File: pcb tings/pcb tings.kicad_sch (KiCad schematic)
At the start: 24 parts, among them SW1 SW_Push, U1 ATmega32U4-A, Y1 16MHz

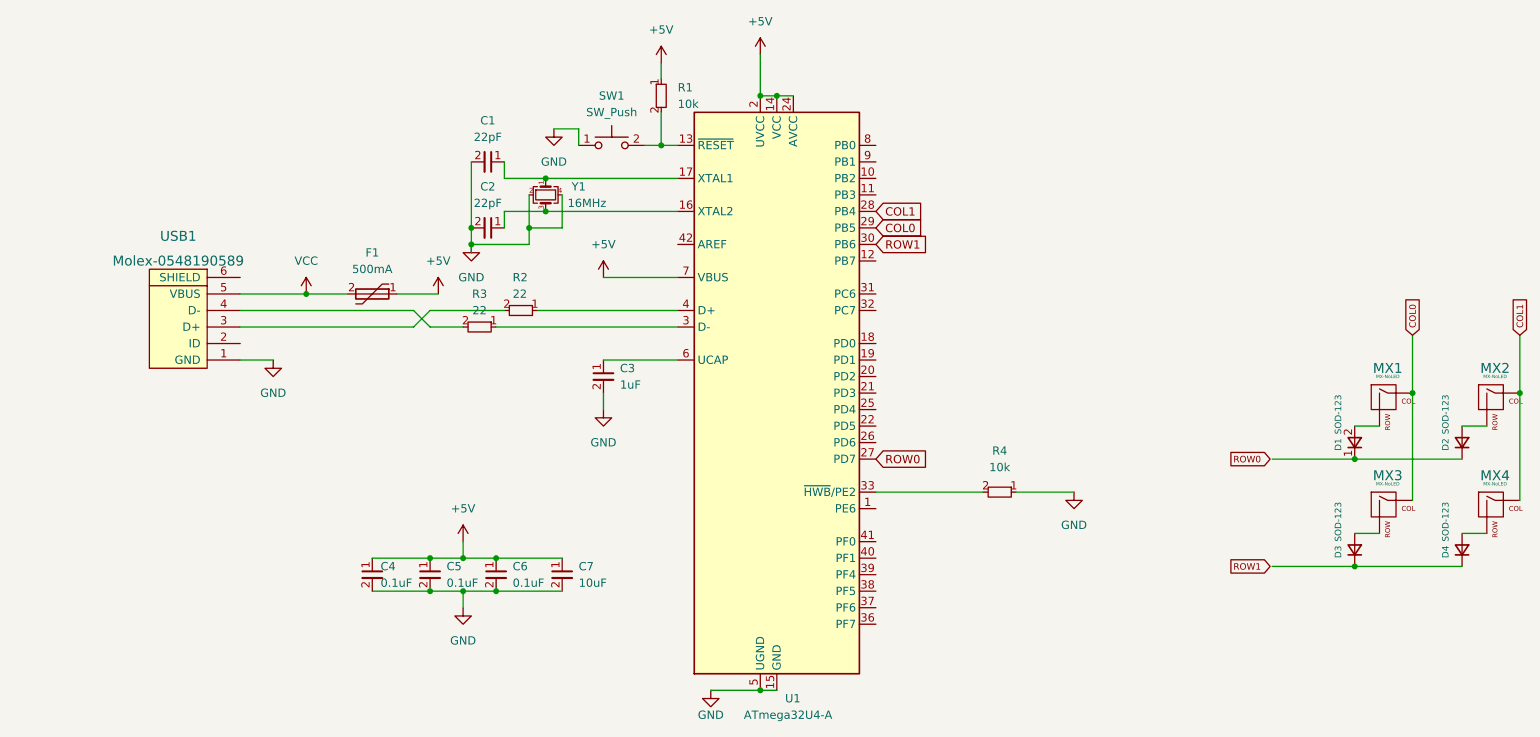
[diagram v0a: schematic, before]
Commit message: Routing
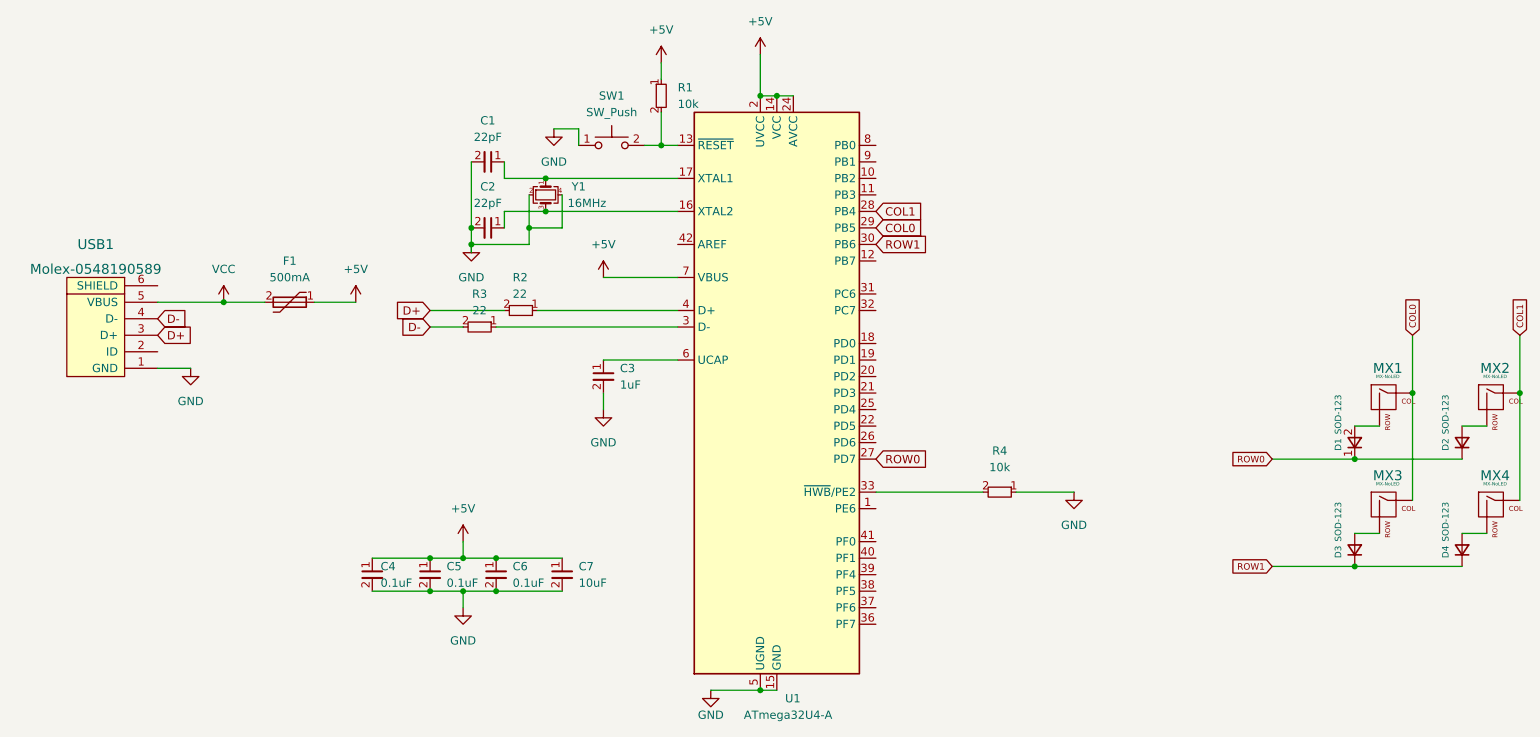
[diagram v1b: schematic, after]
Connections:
- net ROW0: now also D1.1 (K), D2.1 (K)
- net ROW1: now also D3.1 (K), D4.1 (K)
- net D+: now reaches USB1.3 (D+)
- net D+: now also R2.2
- net D-: now reaches USB1.4 (D-)
- net D-: now also R3.2
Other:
- moved on the sheet: F1, USB1
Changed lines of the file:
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@@
   (junction (at 127 48.26) (diameter 0) (color 0 0 0 0)
   )
-  (junction (at 57.15 78.74) (diameter 0) (color 0 0 0 0)
+  (junction (at 44.45 80.01) (diameter 0) (color 0 0 0 0)
   )
   (junction (at 227.33 93.98) (diameter 0) (color 0 0 0 0)
@@
   (junction (at 76.2 124.46) (diameter 0) (color 0 0 0 0)
   )
-  (bus_entry (at 76.2 83.82) (size -2.54 -2.54)
-    (stroke (width 0) (type default) (color 0 0 0 0))
-  )
-  (bus_entry (at 73.66 83.82) (size 2.54 -2.54)
-    (stroke (width 0) (type default) (color 0 0 0 0))
-  )
   (wire (pts (xy 92.71 81.28) (xy 114.3 81.28))
     (stroke (width 0) (type default) (color 0 0 0 0))
@@
     (stroke (width 0) (type default) (color 0 0 0 0))
   )
-  (wire (pts (xy 46.99 78.74) (xy 57.15 78.74))
+  (wire (pts (xy 34.29 80.01) (xy 44.45 80.01))
     (stroke (width 0) (type default) (color 0 0 0 0))
   )
@@
     (stroke (width 0) (type default) (color 0 0 0 0))
   )
-  (wire (pts (xy 46.99 81.28) (xy 73.66 81.28))
-    (stroke (width 0) (type default) (color 0 0 0 0))
-  )
   (wire (pts (xy 111.76 50.8) (xy 111.76 55.88))
     (stroke (width 0) (type default) (color 0 0 0 0))
@@
     (stroke (width 0) (type default) (color 0 0 0 0))
   )
-  (wire (pts (xy 57.15 78.74) (xy 63.5 78.74))
+  (wire (pts (xy 44.45 80.01) (xy 50.8 80.01))
     (stroke (width 0) (type default) (color 0 0 0 0))
   )
@@
     (stroke (width 0) (type default) (color 0 0 0 0))
   )
-  (wire (pts (xy 46.99 83.82) (xy 73.66 83.82))
-    (stroke (width 0) (type default) (color 0 0 0 0))
-  )
   (wire (pts (xy 218.44 120.65) (xy 234.95 120.65))
     (stroke (width 0) (type default) (color 0 0 0 0))
@@
     (stroke (width 0) (type default) (color 0 0 0 0))
   )
-  (wire (pts (xy 71.12 78.74) (xy 77.47 78.74))
+  (wire (pts (xy 58.42 80.01) (xy 64.77 80.01))
     (stroke (width 0) (type default) (color 0 0 0 0))
   )
@@
     (stroke (width 0) (type default) (color 0 0 0 0))
   )
-  (wire (pts (xy 46.99 88.9) (xy 52.07 88.9))
+  (wire (pts (xy 34.29 90.17) (xy 39.37 90.17))
     (stroke (width 0) (type default) (color 0 0 0 0))
   )
@@
   (wire (pts (xy 93.98 60.96) (xy 114.3 60.96))
     (stroke (width 0) (type default) (color 0 0 0 0))
+  )
+  (global_label "D-" (shape input) (at 34.29 82.55 0) (fields_autoplaced)
+    (effects (font (size 1.27 1.27)) (justify left))
+    (property "Intersheet References" "${INTERSHEET_REFS}" (id 0) (at 39.5455 82.4706 0)
+      (effects (font (size 1.27 1.27)) (justify left) hide)
+    )
   )
   (global_label "COL0" (shape input) (at 227.33 85.09 90) (fields_autoplaced)
@@
     )
   )
+  (global_label "D+" (shape input) (at 34.29 85.09 0) (fields_autoplaced)
+    (effects (font (size 1.27 1.27)) (justify left))
+    (property "Intersheet References" "${INTERSHEET_REFS}" (id 0) (at 39.5455 85.0106 0)
+      (effects (font (size 1.27 1.27)) (justify left) hide)
+    )
+  )
   (global_label "ROW0" (shape input) (at 144.78 104.14 0) (fields_autoplaced)
     (effects (font (size 1.27 1.27)) (justify left))
@@
     )
   )
-  (global_label "ROW1" (shape output) (at 199.39 120.65 0) (fields_autoplaced)
-    (effects (font (size 1 1)) (justify left))
-    (property "Intersheet References" "${INTERSHEET_REFS}" (id 0) (at 205.4329 120.5875 0)
-      (effects (font (size 1 1)) (justify left) hide)
-    )
-  )
-  (global_label "ROW0" (shape output) (at 199.39 104.14 0) (fields_autoplaced)
-    (effects (font (size 1 1)) (justify left))
-    (property "Intersheet References" "${INTERSHEET_REFS}" (id 0) (at 205.4329 104.0775 0)
-      (effects (font (size 1 1)) (justify left) hide)
+  (global_label "D-" (shape input) (at 76.2 83.82 180) (fields_autoplaced)
+    (effects (font (size 1.27 1.27)) (justify right))
+    (property "Intersheet References" "${INTERSHEET_REFS}" (id 0) (at 70.9445 83.7406 0)
+      (effects (font (size 1.27 1.27)) (justify right) hide)
+    )
+  )
+  (global_label "ROW1" (shape input) (at 205.74 120.65 180) (fields_autoplaced)
+    (effects (font (size 1 1)) (justify right))
+    (property "Intersheet References" "${INTERSHEET_REFS}" (id 0) (at 199.6971 120.5875 0)
+      (effects (font (size 1 1)) (justify right) hide)
+    )
+  )
+  (global_label "D+" (shape input) (at 76.2 81.28 180) (fields_autoplaced)
+    (effects (font (size 1.27 1.27)) (justify right))
+    (property "Intersheet References" "${INTERSHEET_REFS}" (id 0) (at 70.9445 81.2006 0)
+      (effects (font (size 1.27 1.27)) (justify right) hide)
+    )
+  )
+  (global_label "ROW0" (shape input) (at 205.74 104.14 180) (fields_autoplaced)
+    (effects (font (size 1 1)) (justify right))
+    (property "Intersheet References" "${INTERSHEET_REFS}" (id 0) (at 199.6971 104.0775 0)
+      (effects (font (size 1 1)) (justify right) hide)
     )
   )
@@
     (pin "1")
   )
-  (symbol (lib_id "Device:Polyfuse") (at 67.31 78.74 270) (unit 1)
-    (in_bom yes) (on_board yes) (fields_autoplaced)
-    (property "Reference" "F1" (id 0) (at 67.31 72.39 90))
-    (property "Value" "500mA" (id 1) (at 67.31 74.93 90))
-    (property "Footprint" "Fuse:Fuse_1206_3216Metric" (id 2) (at 62.23 80.01 0)
+  (symbol (lib_id "Device:Polyfuse") (at 54.61 80.01 270) (unit 1)
+    (in_bom yes) (on_board yes) (fields_autoplaced)
+    (property "Reference" "F1" (id 0) (at 54.61 73.66 90))
+    (property "Value" "500mA" (id 1) (at 54.61 76.2 90))
+    (property "Footprint" "Fuse:Fuse_1206_3216Metric" (id 2) (at 49.53 81.28 0)
       (effects (font (size 1.27 1.27)) (justify left) hide)
     )
-    (property "Datasheet" "~" (id 3) (at 67.31 78.74 0)
+    (property "Datasheet" "~" (id 3) (at 54.61 80.01 0)
       (effects (font (size 1.27 1.27)) hide)
     )
@@
     (pin "4")
   )
-  (symbol (lib_id "power:+5V") (at 77.47 78.74 0) (unit 1)
-    (in_bom yes) (on_board yes) (fields_autoplaced)
-    (property "Reference" "#PWR05" (id 0) (at 77.47 82.55 0)
-      (effects (font (size 1.27 1.27)) hide)
-    )
-    (property "Value" "+5V" (id 1) (at 77.47 73.66 0))
-    (property "Footprint" "" (id 2) (at 77.47 78.74 0)
-      (effects (font (size 1.27 1.27)) hide)
-    )
-    (property "Datasheet" "" (id 3) (at 77.47 78.74 0)
-      (effects (font (size 1.27 1.27)) hide)
-    )
-    (pin "1")
-  )
-  (symbol (lib_id "power:VCC") (at 57.15 78.74 0) (unit 1)
-    (in_bom yes) (on_board yes) (fields_autoplaced)
-    (property "Reference" "#PWR04" (id 0) (at 57.15 82.55 0)
-      (effects (font (size 1.27 1.27)) hide)
-    )
-    (property "Value" "VCC" (id 1) (at 57.15 73.66 0))
-    (property "Footprint" "" (id 2) (at 57.15 78.74 0)
-      (effects (font (size 1.27 1.27)) hide)
-    )
-    (property "Datasheet" "" (id 3) (at 57.15 78.74 0)
+  (symbol (lib_id "power:+5V") (at 64.77 80.01 0) (unit 1)
+    (in_bom yes) (on_board yes) (fields_autoplaced)
+    (property "Reference" "#PWR05" (id 0) (at 64.77 83.82 0)
+      (effects (font (size 1.27 1.27)) hide)
+    )
+    (property "Value" "+5V" (id 1) (at 64.77 74.93 0))
+    (property "Footprint" "" (id 2) (at 64.77 80.01 0)
+      (effects (font (size 1.27 1.27)) hide)
+    )
+    (property "Datasheet" "" (id 3) (at 64.77 80.01 0)
+      (effects (font (size 1.27 1.27)) hide)
+    )
+    (pin "1")
+  )
+  (symbol (lib_id "power:VCC") (at 44.45 80.01 0) (unit 1)
+    (in_bom yes) (on_board yes) (fields_autoplaced)
+    (property "Reference" "#PWR04" (id 0) (at 44.45 83.82 0)
+      (effects (font (size 1.27 1.27)) hide)
+    )
+    (property "Value" "VCC" (id 1) (at 44.45 74.93 0))
+    (property "Footprint" "" (id 2) (at 44.45 80.01 0)
+      (effects (font (size 1.27 1.27)) hide)
+    )
+    (property "Datasheet" "" (id 3) (at 44.45 80.01 0)
       (effects (font (size 1.27 1.27)) hide)
     )
@@
     (pin "2")
   )
-  (symbol (lib_id "random-keyboard-parts:Molex-0548190589") (at 39.37 83.82 90) (unit 1)
-    (in_bom yes) (on_board yes) (fields_autoplaced)
-    (property "Reference" "USB1" (id 0) (at 37.465 69.85 90)
+  (symbol (lib_id "random-keyboard-parts:Molex-0548190589") (at 26.67 85.09 90) (unit 1)
+    (in_bom yes) (on_board yes) (fields_autoplaced)
+    (property "Reference" "USB1" (id 0) (at 24.765 71.12 90)
       (effects (font (size 1.524 1.524)))
     )
-    (property "Value" "Molex-0548190589" (id 1) (at 37.465 73.66 90)
+    (property "Value" "Molex-0548190589" (id 1) (at 24.765 74.93 90)
       (effects (font (size 1.524 1.524)))
     )
-    (property "Footprint" "random-keyboard-parts:Molex-0548190589" (id 2) (at 39.37 83.82 0)
-      (effects (font (size 1.524 1.524)) hide)
-    )
-    (property "Datasheet" "" (id 3) (at 39.37 83.82 0)
+    (property "Footprint" "random-keyboard-parts:Molex-0548190589" (id 2) (at 26.67 85.09 0)
+      (effects (font (size 1.524 1.524)) hide)
+    )
+    (property "Datasheet" "" (id 3) (at 26.67 85.09 0)
       (effects (font (size 1.524 1.524)) hide)
     )
@@
     (pin "2")
   )
-  (symbol (lib_id "power:GND") (at 52.07 88.9 0) (unit 1)
-    (in_bom yes) (on_board yes) (fields_autoplaced)
-    (property "Reference" "#PWR07" (id 0) (at 52.07 95.25 0)
-      (effects (font (size 1.27 1.27)) hide)
-    )
-    (property "Value" "GND" (id 1) (at 52.07 93.98 0))
-    (property "Footprint" "" (id 2) (at 52.07 88.9 0)
-      (effects (font (size 1.27 1.27)) hide)
-    )
-    (property "Datasheet" "" (id 3) (at 52.07 88.9 0)
-      (effects (font (size 1.27 1.27)) hide)
-    )
+  (symbol (lib_id "power:GND") (at 39.37 90.17 0) (unit 1)
+    (in_bom yes) (on_board yes) (fields_autoplaced)
+    (property "Reference" "#PWR07" (id 0) (at 39.37 96.52 0)
+      (effects (font (size 1.27 1.27)) hide)
+    )
+    (property "Value" "GND" (id 1) (at 39.37 95.25 0))
+    (property "Footprint" "" (id 2) (at 39.37 90.17 0)
+      (effects (font (size 1.27 1.27)) hide)
+    )
+    (property "Datasheet" "" (id 3) (at 39.37 90.17 0)
+      (effects (font (size 1.27 1.27)) hide)
+    )
